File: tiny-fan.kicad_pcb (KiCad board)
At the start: 2 copper layers, 56.4 x 51.8 mm, 69 parts, among them Q1 BSS138, Q2 BSS138, Q3 BSS138, Q4 BSS138, Q5 BSS138, Q6 BSS138, Q7 BSS138, U1 L7812, U2 tiny2040

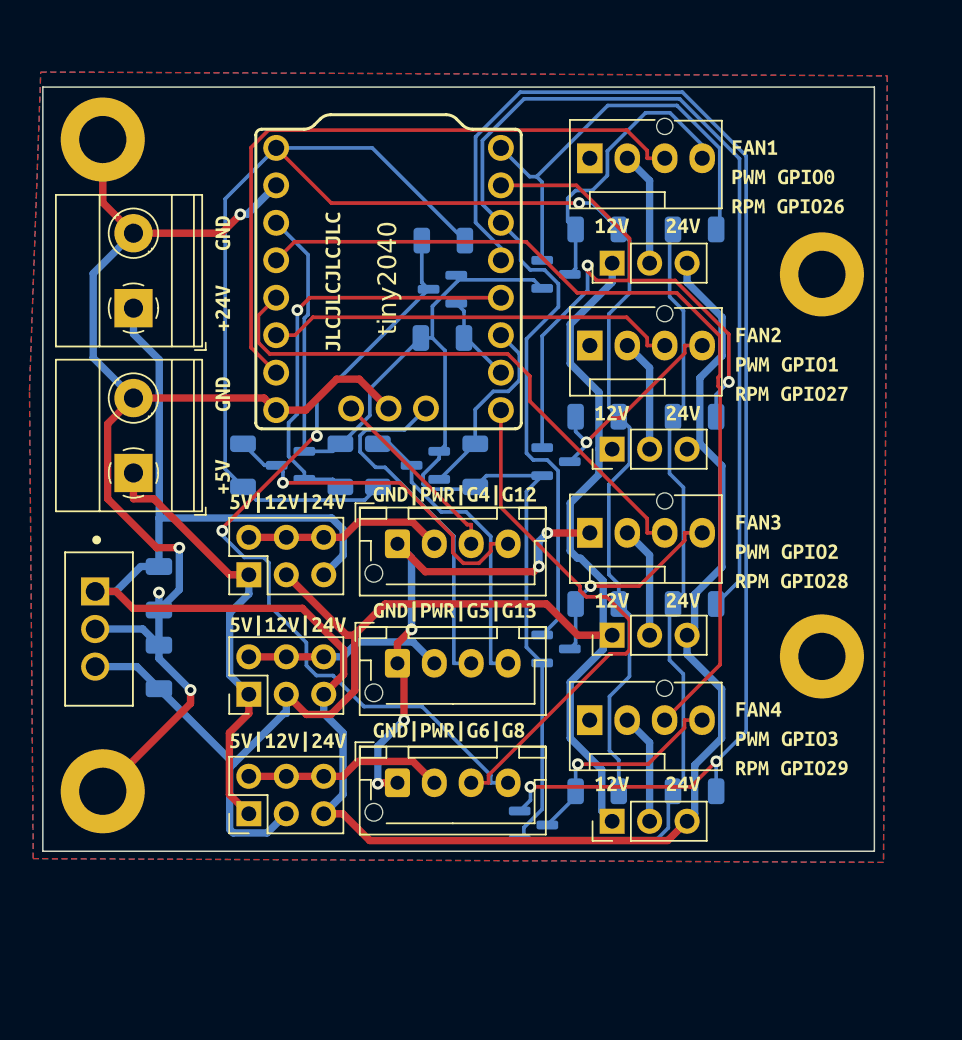
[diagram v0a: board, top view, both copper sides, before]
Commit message: version 2
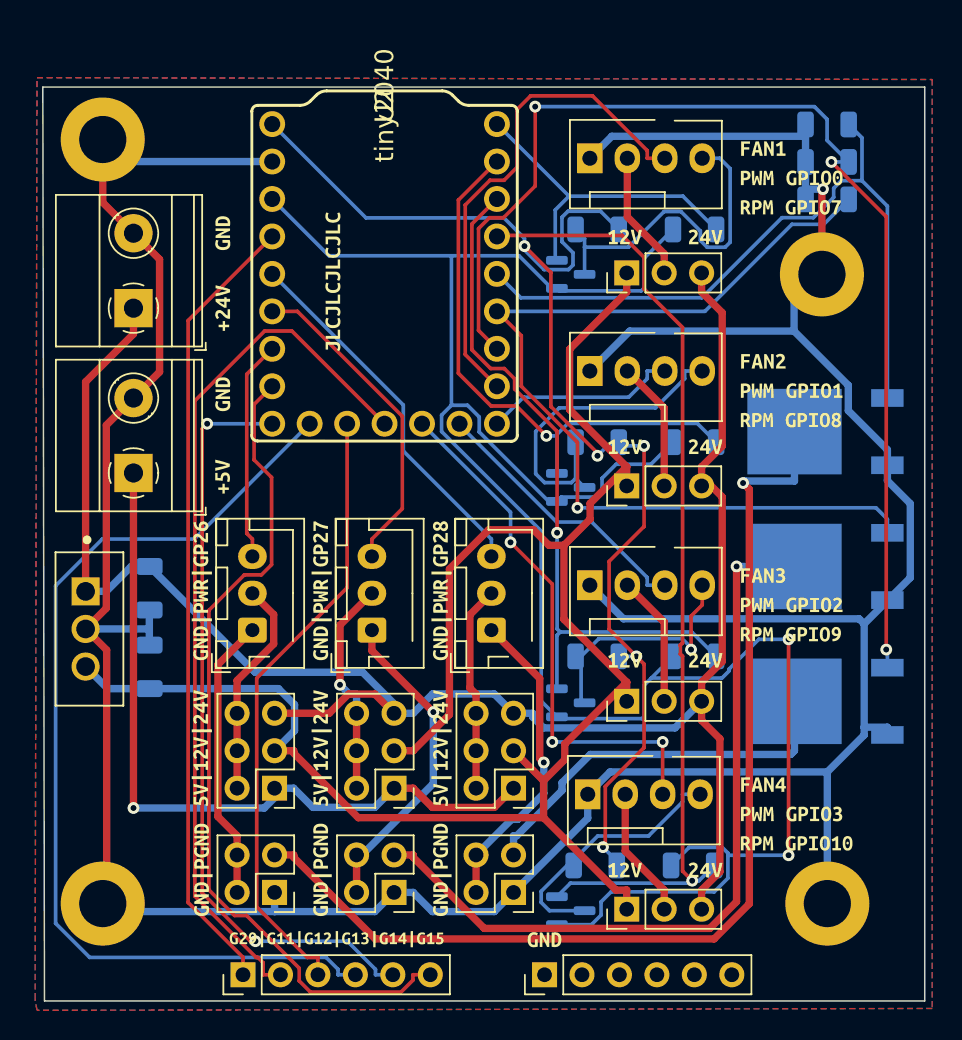
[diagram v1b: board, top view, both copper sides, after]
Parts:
- removed Q5, Q6, Q7: BSS138, Package_TO_SOT_SMD:SOT-23
- removed R10, R11, R12, R13, R14, R9: 10K, Resistor_SMD:R_1206_3216Metric
- removed kibuzzard-62F42A54: G***, kibuzzard-62F42A54
- removed kibuzzard-62F42B83: G***, kibuzzard-62F42B83
- removed kibuzzard-62F42B98: G***, kibuzzard-62F42B98
- removed kibuzzard-62F42BB7: G***, kibuzzard-62F42BB7
- removed kibuzzard-62F4A92A: G***, kibuzzard-62F4A92A
- removed kibuzzard-62F4E423: G***, kibuzzard-62F4E423
- removed kibuzzard-62F4E43D: G***, kibuzzard-62F4E43D
- removed kibuzzard-62F4E44F: G***, kibuzzard-62F4E44F
- added J1: Conn_02x02_Odd_Even, Connector_PinHeader_2.54mm:PinHeader_2x02_P2.54mm_Vertical, F.Cu at (29.3, 68.6)
- added J2: Conn_02x02_Odd_Even, Connector_PinHeader_2.54mm:PinHeader_2x02_P2.54mm_Vertical, F.Cu at (37.4, 68.6)
- added J3: Conn_02x02_Odd_Even, Connector_PinHeader_2.54mm:PinHeader_2x02_P2.54mm_Vertical, F.Cu at (45.5, 68.6)
- added J4: Conn_01x06_Male, Connector_PinHeader_2.54mm:PinHeader_1x06_P2.54mm_Vertical, F.Cu at (27.2, 74.2)
- added J5: Conn_01x06_Male, Connector_PinHeader_2.54mm:PinHeader_1x06_P2.54mm_Vertical, F.Cu at (47.6, 74.2)
- added Q10: wsf3085, Package_TO_SOT_SMD:TO-252-2, B.Cu at (66.7, 55.6)
- added Q8: wsf3085, Package_TO_SOT_SMD:TO-252-2, B.Cu at (66.7, 37.3)
- added Q9: wsf3085, Package_TO_SOT_SMD:TO-252-2, B.Cu at (66.7, 46.5)
- added R15: 10K, Resistor_SMD:R_1206_3216Metric, B.Cu at (66.8, 16.5)
- added R16: 10K, Resistor_SMD:R_1206_3216Metric, B.Cu at (66.8, 21.6)
- added R17: 10K, Resistor_SMD:R_1206_3216Metric, B.Cu at (66.8, 19.1)
- added kibuzzard-62F894BF: G***, kibuzzard-62F894BF, F.Cu at (24.4, 67.1)
- added kibuzzard-62F894CE: G***, kibuzzard-62F894CE, F.Cu at (32.5, 67.1)
- added kibuzzard-62F894DE: G***, kibuzzard-62F894DE, F.Cu at (40.6, 67.1)
- added kibuzzard-630F902C: G***, kibuzzard-630F902C, F.Cu at (64.4, 20.1)
- added kibuzzard-630F9081: G***, kibuzzard-630F9081, F.Cu at (64.4, 34.6)
- added kibuzzard-630F9093: G***, kibuzzard-630F9093, F.Cu at (64.4, 49.1)
- added kibuzzard-630F90A1: G***, kibuzzard-630F90A1, F.Cu at (64.7, 63.3)
- added kibuzzard-630F9163: G***, kibuzzard-630F9163, F.Cu at (24.4, 48.1)
- added kibuzzard-630F9189: G***, kibuzzard-630F9189, F.Cu at (32.5, 48.1)
- added kibuzzard-630F9193: G***, kibuzzard-630F9193, F.Cu at (40.6, 48.1)
- added kibuzzard-630F922D: G***, kibuzzard-630F922D, F.Cu at (33.5, 71.8)
- added kibuzzard-63104730: G***, kibuzzard-63104730, F.Cu at (47.6, 71.8)
- added kibuzzard-631047F8: G***, kibuzzard-631047F8, B.Cu at (36.2, 40.6)
- AUX1, AUX2, AUX3: value Conn_01x04 -> Conn_01x03; footprint Connector_JST:JST_XH_B4B-XH-AM_1x04_P2.50mm_Vertical -> Connector_JST:JST_XH_B3B-XH-AM_1x03_P2.50mm_Vertical
- U2: footprint _my_own:tiny2040 -> _my_own:rp2040_zero
- moved AUX3PWR1 18.0 mm to (45.5, 61.5), turned to 180 degrees
- moved kibuzzard-62F42661 17.6 mm to (24.4, 58.8), turned to 90 degrees
- moved REF4 16.8 mm to (66.8, 69.3)
- moved AUX1PWR1 14.6 mm to (29.3, 61.5), turned to 180 degrees
- moved AUX3 12.2 mm to (44.0, 50.8), turned to 90 degrees
- moved AUX2PWR1 11.7 mm to (37.4, 61.5), turned to 180 degrees
- moved AUX1 11.4 mm to (27.8, 50.8), turned to 90 degrees
- moved kibuzzard-62F426613 10.4 mm to (40.6, 58.8), turned to 90 degrees
- moved kibuzzard-62F426612 8.61 mm to (32.5, 58.8), turned to 90 degrees
- moved REF2 7.62 mm to (17.7, 69.3)
- moved Q4 6.33 mm to (49.4, 69.8)
- moved FAN4PWR1 6.04 mm to (53.2, 69.7)
- moved kibuzzard-62F4288845 6.03 mm to (58.5, 67.1)
- moved kibuzzard-62F4287AC 5.90 mm to (53.1, 67.1)
- moved R5 5.03 mm to (57.7, 66.8)
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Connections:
- AUX1 pad 1: GND -> AUX1GND
- AUX1 pad 3: AUX1RPM -> AUX1DATA
- AUX2 pad 1: GND -> AUX2GND
- AUX2 pad 3: AUX2RPM -> AUX2DATA
- AUX3 pad 1: GND -> AUX3GND
- AUX3 pad 3: AUX3RPM -> AUX3DATA
- U2 pad 1: +5VA -> FAN2PWM
- U2 pad 10: AUX3PWM -> FAN4RPM
- U2 pad 11: AUX2PWM -> AUX4
- U2 pad 12: AUX1PWM -> AUX5
- U2 pad 13: FAN4PWM -> AUX6
- U2 pad 14: FAN3PWM -> AUX7
- U2 pad 15: FAN2PWM -> AUX8
- U2 pad 2: GND -> FAN3PWM
- U2 pad 3: +3V3 -> FAN4PWM
- U2 pad 4: FAN4RPM -> AUX1PWM
- U2 pad 5: FAN3RPM -> AUX2PWM
- U2 pad 6: FAN2RPM -> AUX3PWM
- U2 pad 8: GND -> FAN2RPM
- U2 pad 9: AUX3RPM -> FAN3RPM
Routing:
- net GND: track 126.5 -> 244.8 mm, vias 9 -> 1
- net AUX3PWM: track 6.05 -> 79.8 mm, vias 0 -> 3
- net AUX1MPWR: track 0.00 -> 71.2 mm, vias 0 -> 1
- net AUX6: track 0.00 -> 66.7 mm
- net AUX4: track 0.00 -> 59.5 mm
- net AUX8: track 0.00 -> 56.7 mm
- net Net-(AUX3-Pad4): track 55.3 -> 0.00 mm, vias 2 -> 0
- net AAUX1: track 0.00 -> 54.0 mm
- net AUX2MPWR: track 0.00 -> 52.8 mm, vias 0 -> 1
- net AUX7: track 0.00 -> 51.8 mm, vias 0 -> 2
- net AUX2PWM: track 13.2 -> 64.8 mm, vias 0 -> 1
- net AUX5: track 0.00 -> 42.0 mm
- net FAN3PWM: track 90.2 -> 48.3 mm, vias 0 -> 1
- net AUX3RPM: track 35.5 -> 0.00 mm
- net +5VA: track 117.3 -> 86.6 mm, vias 1 -> 5
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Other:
- board size 56.4 x 51.8 mm -> 59.8 x 62 mm
